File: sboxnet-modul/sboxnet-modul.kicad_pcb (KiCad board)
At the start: 2 copper layers, 49.6 x 46.2 mm, 33 parts, among them J2 Conn_02x03_Odd_Even, J4 8P8C, J5 8P8C, J6 sboxnet-buchse_2x17, SW1 SW_Push, U1  3.3V MCP1703A-3302_SOT223, U2  5V MCP1703A-5002_SOT223, U3 SN65HVD230, U4 ATxmega128A4U-AU, Y1 16MHz

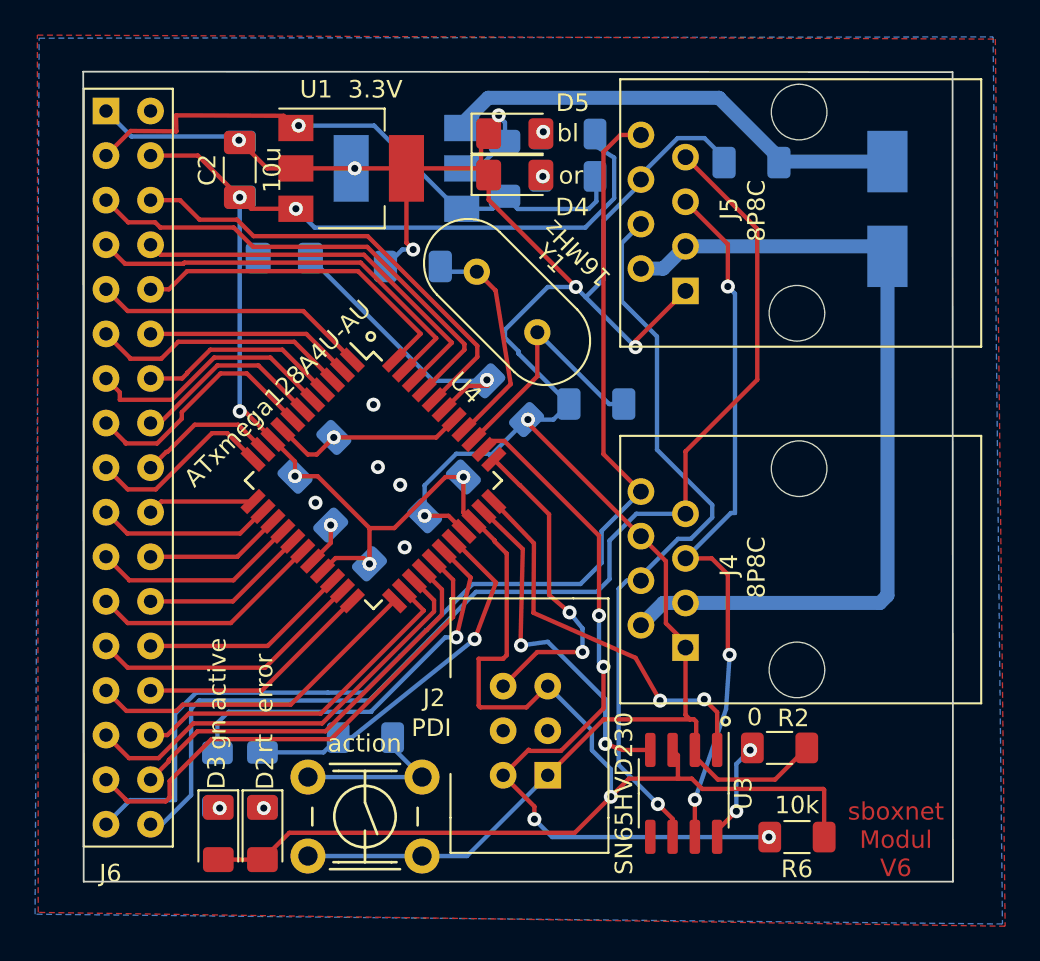
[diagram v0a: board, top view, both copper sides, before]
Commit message: sboxnet Modul v6 fertig
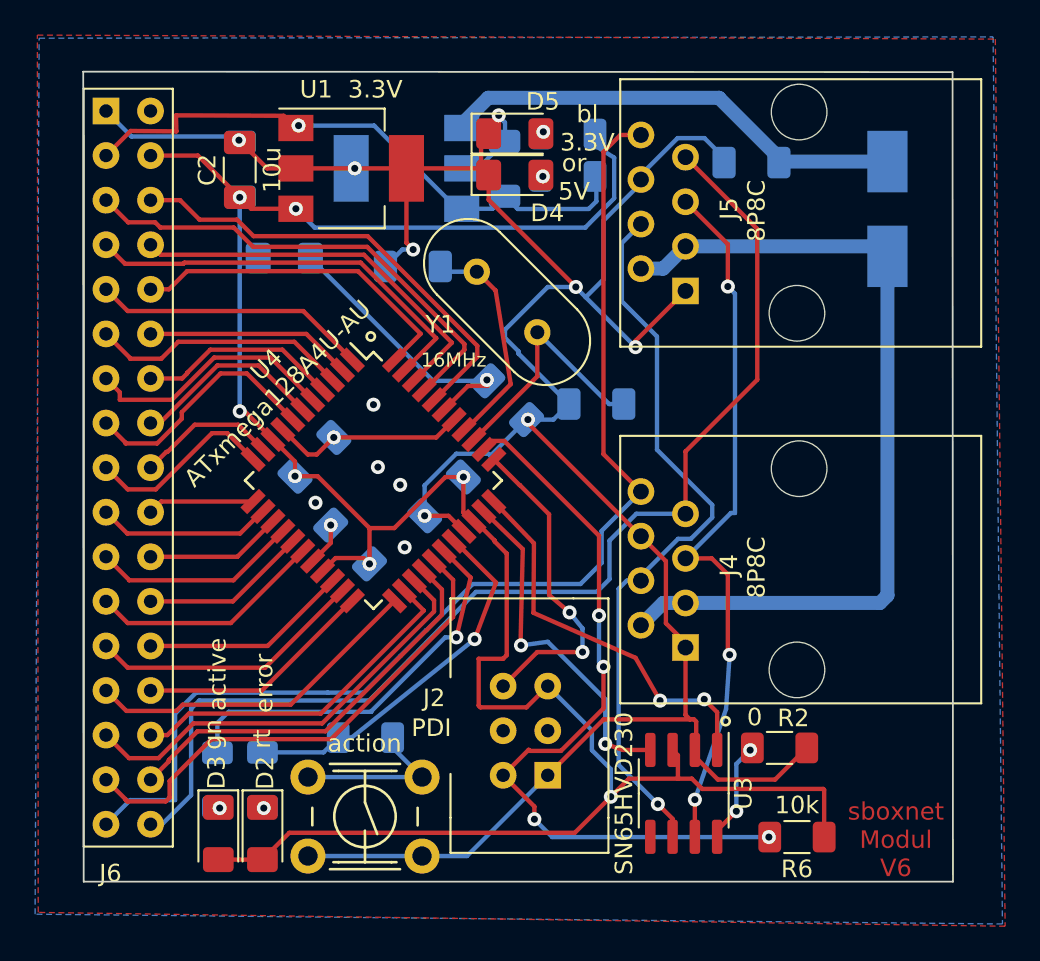
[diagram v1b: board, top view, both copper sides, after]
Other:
- board text added: "bl 3.3V"
- board text added: "or 5V"
- board text removed: "bl"
- board text removed: "or"
